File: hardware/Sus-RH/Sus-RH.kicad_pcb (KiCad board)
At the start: 2 copper layers, 48.5 x 61 mm, 35 parts, among them J2 53307-2471, J3 MX150_02x06_RightAngle, J4 Conn_01x06, J5 Conn_01x06, U1 TLV9002QDRQ1

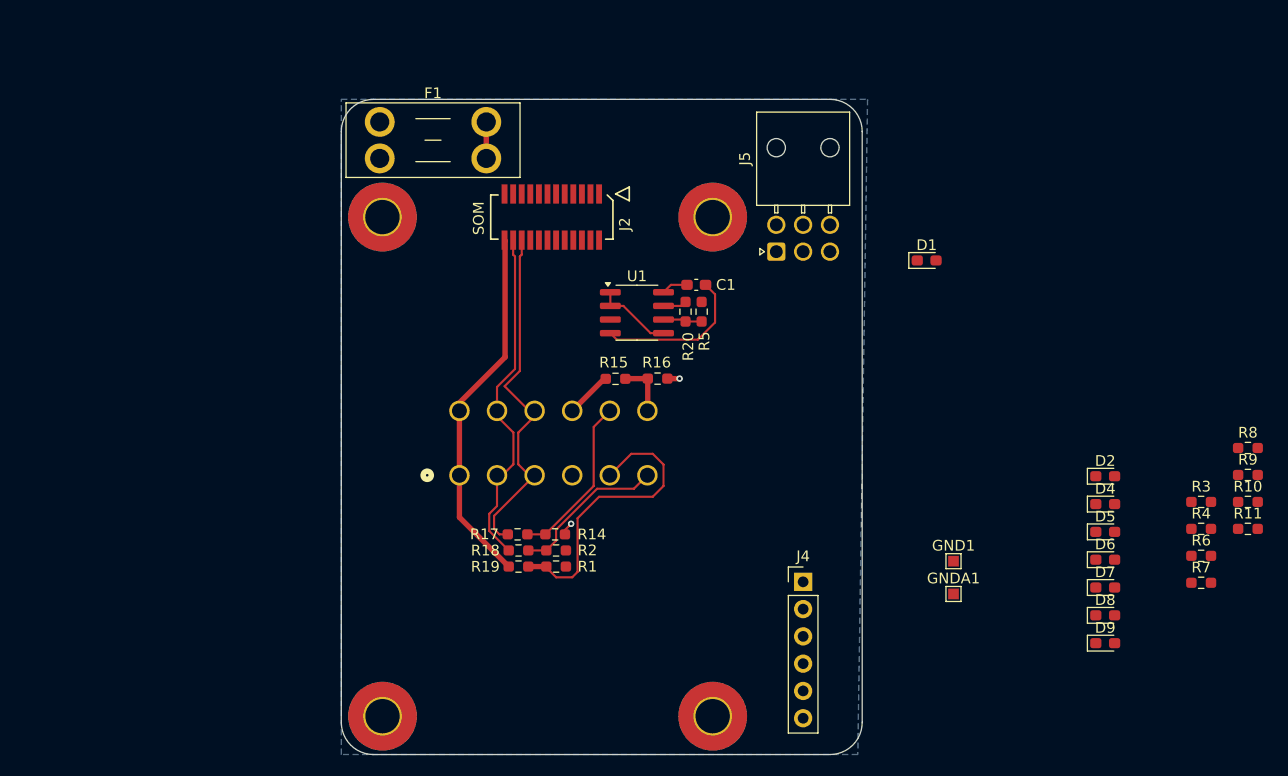
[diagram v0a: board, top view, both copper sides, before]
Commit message: layout finished, need to add some more silkscreen + ready for review!
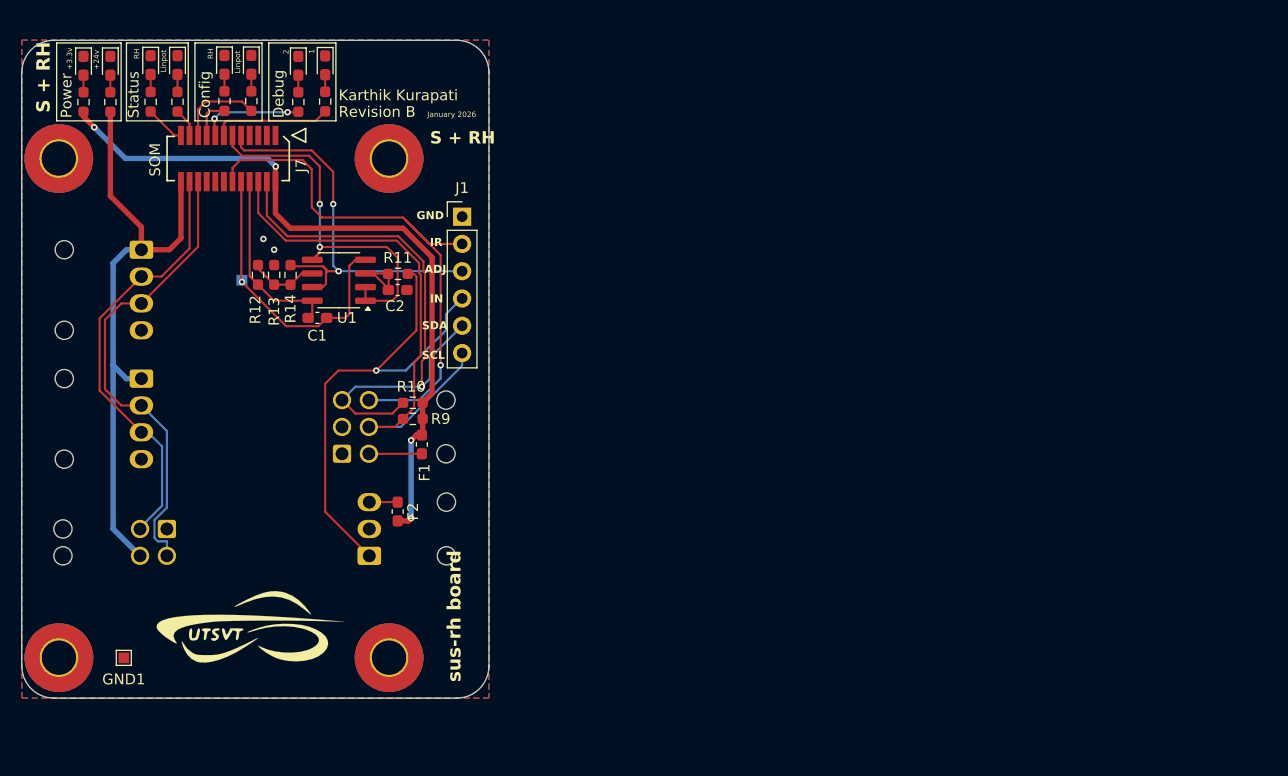
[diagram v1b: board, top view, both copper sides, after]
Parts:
- removed D9: LED, LED_SMD:LED_0603_1608Metric_Pad1.05x0.95mm_HandSolder
- removed R15, R16, R17, R18, R19: 0, Resistor_SMD:R_0603_1608Metric_Pad0.98x0.95mm_HandSolder
- removed R20: R, Resistor_SMD:R_0603_1608Metric_Pad0.98x0.95mm_HandSolder
- added C2: 1uF, Capacitor_SMD:C_0603_1608Metric_Pad1.08x0.95mm_HandSolder, F.Cu at (61.2, 39.8)
- added D3: LED, LED_SMD:LED_0603_1608Metric_Pad1.05x0.95mm_HandSolder, F.Cu at (38.2, 18.8)
- added F2: 500mA, Fuse:Fuse_0603_1608Metric_Pad1.05x0.95mm_HandSolder, F.Cu at (61.2, 60.4)
- added G***: LHRs_LOGO, UTSVT_Logos:LHRs_LOGO, F.Cu at (62.8, 19.2)
- added G***: LOGO, UTSVT_Logos:UTSVT_Logo_Symbol, F.Cu at (47.2, 71.2)
- added J1: Conn_01x06, Connector_PinHeader_2.54mm:PinHeader_1x06_P2.54mm_Vertical, F.Cu at (67.2, 32.9)
- added J6: Conn_01x03, Connector_Molex:Molex_Nano-Fit_105313-xx03_1x03_P2.50mm_Horizontal, B.Cu at (58.6, 64.5)
- added J7: 53307-2471, UTSVT_Connectors:PeripheralSOM, F.Cu at (45.5, 27.5)
- added R12: 4.7k, Resistor_SMD:R_0603_1608Metric_Pad0.98x0.95mm_HandSolder, F.Cu at (48.2, 38.3)
- added R13: 1k, Resistor_SMD:R_0603_1608Metric_Pad0.98x0.95mm_HandSolder, F.Cu at (49.8, 38.3)
- F1: footprint Fuse:Fuseholder_Blade_Mini_Keystone_3568 -> Fuse:Fuse_0603_1608Metric_Pad1.05x0.95mm_HandSolder
- GNDA1, J5: moved to B.Cu
- J2: value 53307-2471 -> Conn_01x04; footprint UTSVT_Connectors:PeripheralSOM -> Connector_Molex:Molex_Nano-Fit_105314-xx04_2x02_P2.50mm_Horizontal; moved to B.Cu
- J3: value MX150_02x06_RightAngle -> Conn_01x04; footprint UTSVT_Connectors:MX150_02x06_RightAngle -> Connector_Molex:Molex_Nano-Fit_105313-xx04_1x04_P2.50mm_Horizontal
- J4: value Conn_01x06 -> Conn_01x04; footprint Connector_PinHeader_2.54mm:PinHeader_1x06_P2.54mm_Vertical -> Connector_Molex:Molex_Nano-Fit_105313-xx04_1x04_P2.50mm_Horizontal; moved to B.Cu
- R1, R2: value 0 -> 1k
- R10, R11, R9: value 1k -> 4.7k
- R3: value 4.7k -> 1k
- R4, R6, R7: value 120 -> 1k
- R5: value R -> 1k
- moved R6 112.3 mm to (32.0, 22.2), turned to 90 degrees
- moved R4 109.1 mm to (34.5, 22.2), turned to 90 degrees
- moved D6 105.7 mm to (32.0, 18.9), turned to -90 degrees
- moved R3 104.7 mm to (38.2, 22.2), turned to 90 degrees
- moved D4 101.2 mm to (34.5, 18.9), turned to -90 degrees
- moved D5 96.7 mm to (40.8, 18.8), turned to -90 degrees
- moved R7 95.2 mm to (52.0, 22.2), turned to 90 degrees
- moved R8 91.8 mm to (54.5, 22.2), turned to 90 degrees
- moved D7 89.5 mm to (52.0, 18.9), turned to -90 degrees
- moved D8 88.9 mm to (54.5, 18.8), turned to -90 degrees
- moved D2 88.2 mm to (47.6, 18.8), turned to -90 degrees
- moved R11 82.6 mm to (61.3, 38.2), turned to 180 degrees
- moved R10 78.3 mm to (62.7, 50.2), turned to 180 degrees
- moved R9 77.9 mm to (62.7, 51.8), turned to 180 degrees
- moved GND1 77.8 mm to (35.8, 74.0), turned to -90 degrees
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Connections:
- F1 pad 1: Net-(J2-+3.3v) -> Net-(J5-Pin_4)
- J2 pad 2: Net-(J2-+3.3v) -> /CAN_-
- J2 pad 3: GND -> /CAN_+
- J2 pad 4: /SDA -> +24V
- J4 pad 1: GND -> +24V
- J4 pad 2: /IR_INTER -> /CAN_-
- J4 pad 3: /linpot_adj -> /CAN_+
- J4 pad 4: /linpot_in -> GND
- J5 pad 1: unconnected-(J5-Pin_1-Pad1) -> GND
- J5 pad 4: +3.3V -> Net-(J5-Pin_4)
- R1 pad 1: /Gen_1 -> /RHConfig
- R1 pad 2: +3.3V -> Net-(D1-A)
- R10 pad 1: /SusConfig -> +3.3V
- R10 pad 2: Net-(D7-A) -> /SDA
- R11 pad 1: /Debug1 -> /linpot_in
- R11 pad 2: Net-(D9-A) -> Net-(U1A-+)
- R14 pad 1: /Gen_3 -> Net-(U1B--)
- R14 pad 2: GND -> /linpot_adj
- R2 pad 1: /Gen_2 -> /SusConfig
- R2 pad 2: /linpot_in -> Net-(D2-A)
- R3 pad 1: +24V -> /RH_STATUS
- R3 pad 2: Net-(D1-A) -> Net-(D3-A)
- R4 pad 1: +3.3V -> +24V
- R4 pad 2: Net-(D2-A) -> Net-(D4-A)
- R5 pad 1: Net-(U1B--) -> /LINPOT_STATUS
- R5 pad 2: GND -> Net-(D5-A)
- R6 pad 1: /RH_STATUS -> +3.3V
- R6 pad 2: Net-(D4-A) -> Net-(D6-A)
- R7 pad 1: /LINPOT_STATUS -> /Debug2
- R7 pad 2: Net-(D5-A) -> Net-(D7-A)
- R8 pad 1: /RHConfig -> /Debug1
- R8 pad 2: Net-(D6-A) -> Net-(D8-A)
- R9 pad 1: /Debug2 -> +3.3V
- R9 pad 2: Net-(D8-A) -> /SCL
- U1 pad 3: /linpot_in -> Net-(U1A-+)
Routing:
- net +3.3V: track 3.40 -> 67.7 mm, vias 0 -> 4
- net /SDA: track 0.00 -> 53.1 mm, vias 0 -> 1
- net /IR_INTER: track 0.00 -> 51.9 mm, vias 0 -> 1
- net /SCL: track 0.00 -> 50.8 mm
- net /linpot_in: track 0.00 -> 46.1 mm, vias 0 -> 1
- net /linpot_adj: track 2.20 -> 39.9 mm, vias 0 -> 2
- net /linpot_out: track 7.27 -> 35.9 mm, vias 0 -> 2
- net /Gen_1: track 27.7 -> 0.00 mm
- net +24V: track 34.6 -> 58.0 mm
- net /Gen_3: track 15.7 -> 0.00 mm
- net VDDA: track 2.47 -> 18.0 mm
- net /Gen_2: track 14.6 -> 0.00 mm
- net GNDA: track 14.5 -> 28.1 mm, vias 0 -> 1
- net /CAN_-: track 33.5 -> 45.1 mm
- net /Debug1: track 0.00 -> 11.0 mm
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- added copper zone on F.Cu, net GND
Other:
- board size 48.5 x 61 mm -> 43.5 x 61.2 mm
- board text added: "+24v"
- board text added: "+3.3v"
- board text added: "1"
- board text added: "2"
- board text added: "ADJ"
- board text added: "Config"
- board text added: "Debug"
- board text added: "GND"
- board text added: "IN"
- board text added: "IR"
- board text added: "January 2026"
- board text added: "Karthik Kurapati"
- board text added: "Linpot"
- board text added: "Power"
- board text added: "RH"
- board text added: "Revision B"
- board text added: "S + RH"
- board text added: "SCL"
- board text added: "SDA"
- board text added: "Status"
- board text added: "sus-rh board"
